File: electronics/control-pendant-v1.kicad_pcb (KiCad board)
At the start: 2 copper layers, 68.7 x 66 mm, 63 parts, among them J1 22-28-4034, J18 M20-7821042, J2 22-28-4034, J3 22-28-4034, J4 1727010, J5 22-28-4034, J6 USB_C_Receptacle_USB2.0, J7 22-28-4034, Q1 MMSS8050-H-TP, Q2 MMSS8050-H-TP, Q3 SQ2361AEES-T1_GE3, Q4 SQ2361AEES-T1_GE3, U1 CP2102N-A02-GQFN24R, U2 ESP32-S3-WROOM-1-N8R8, U4 LT8619, U5 BX0033

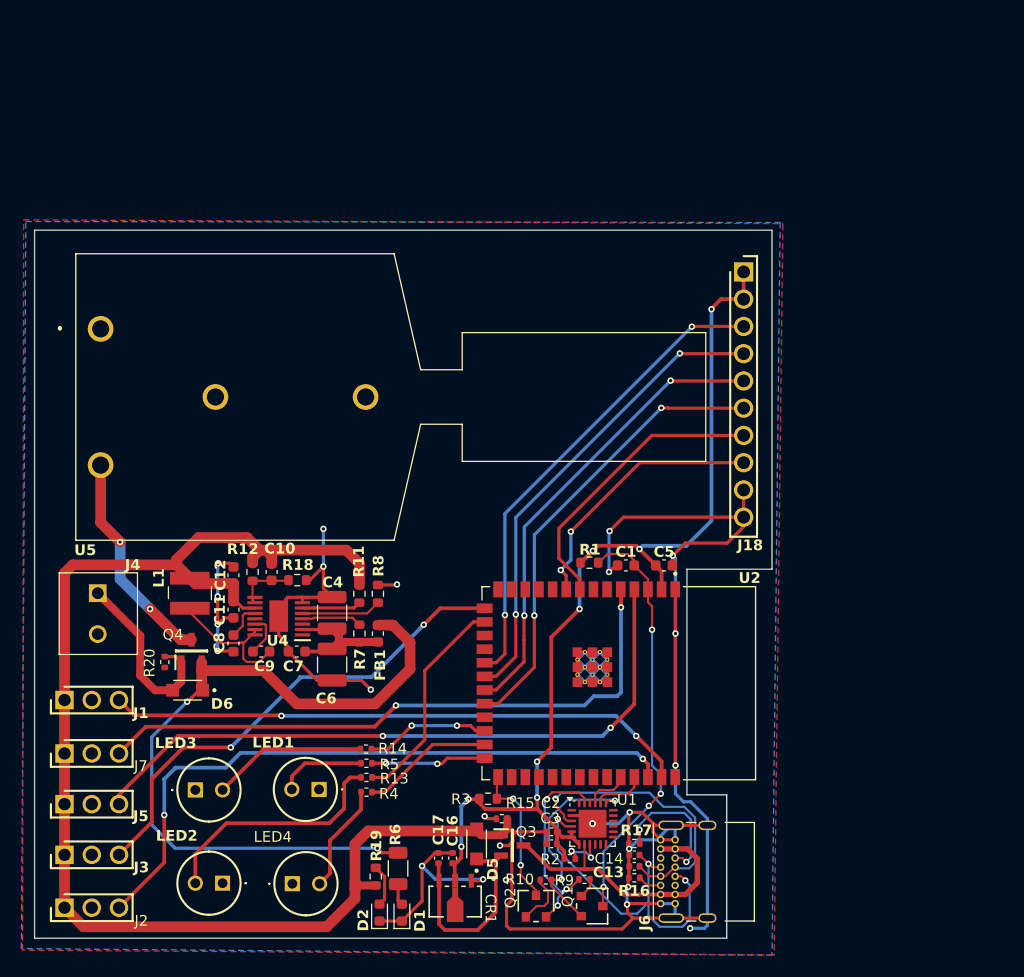
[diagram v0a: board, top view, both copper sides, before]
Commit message: 05/01/2025 Final Commit
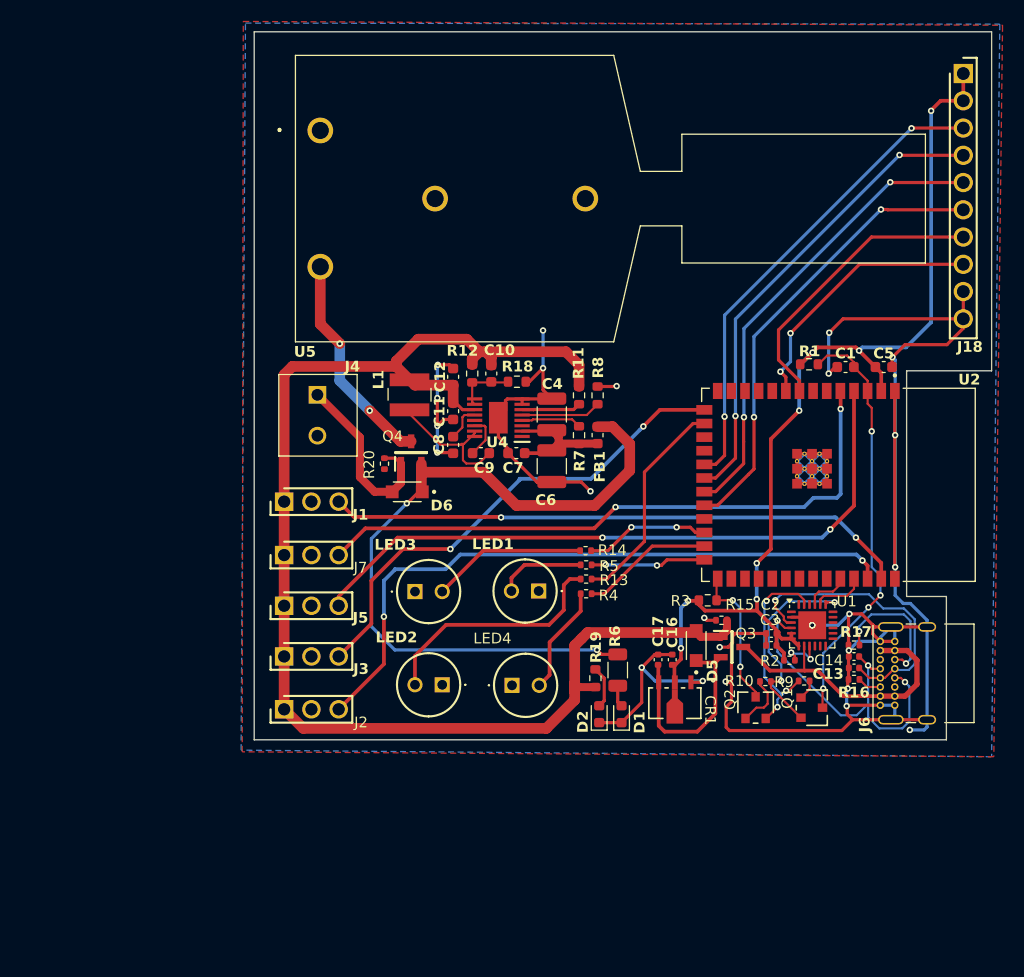
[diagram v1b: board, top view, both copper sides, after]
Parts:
- moved C10 27.6 mm to (60.1, 57.6)
- moved C11 27.6 mm to (56.5, 61.1)
- moved C12 27.6 mm to (56.5, 57.9)
- moved C13 27.6 mm to (93.9, 85.0)
- moved C14 27.6 mm to (93.9, 83.9)
- moved C16 27.6 mm to (77.0, 84.2)
- moved C17 27.6 mm to (75.6, 84.2)
- moved C4 27.6 mm to (65.7, 61.4)
- moved CR1 27.6 mm to (77.2, 88.3)
- moved D1 27.6 mm to (72.2, 89.3)
- moved D6 27.6 mm to (52.3, 68.6)
- moved J1 27.6 mm to (40.8, 69.5)
- moved J2 27.6 mm to (40.8, 88.8)
- moved J3 27.6 mm to (40.8, 83.9)
- moved J5 27.6 mm to (40.8, 79.2)
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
